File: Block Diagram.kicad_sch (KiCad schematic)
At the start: 0 parts

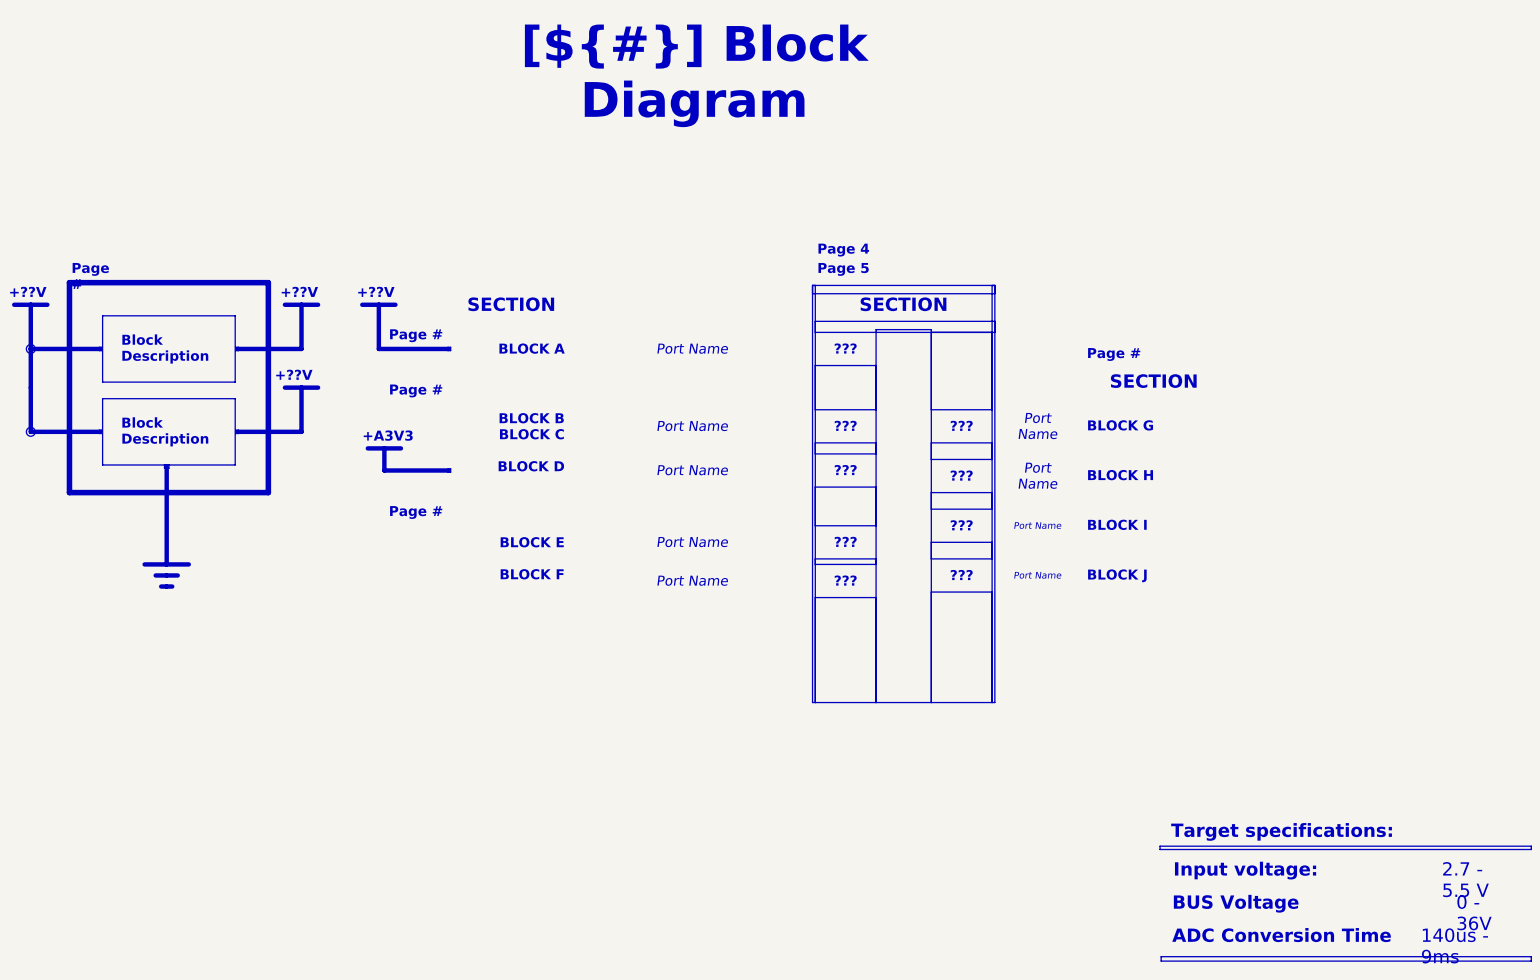
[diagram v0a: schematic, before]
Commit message: Outputs generated, ready for prototyping
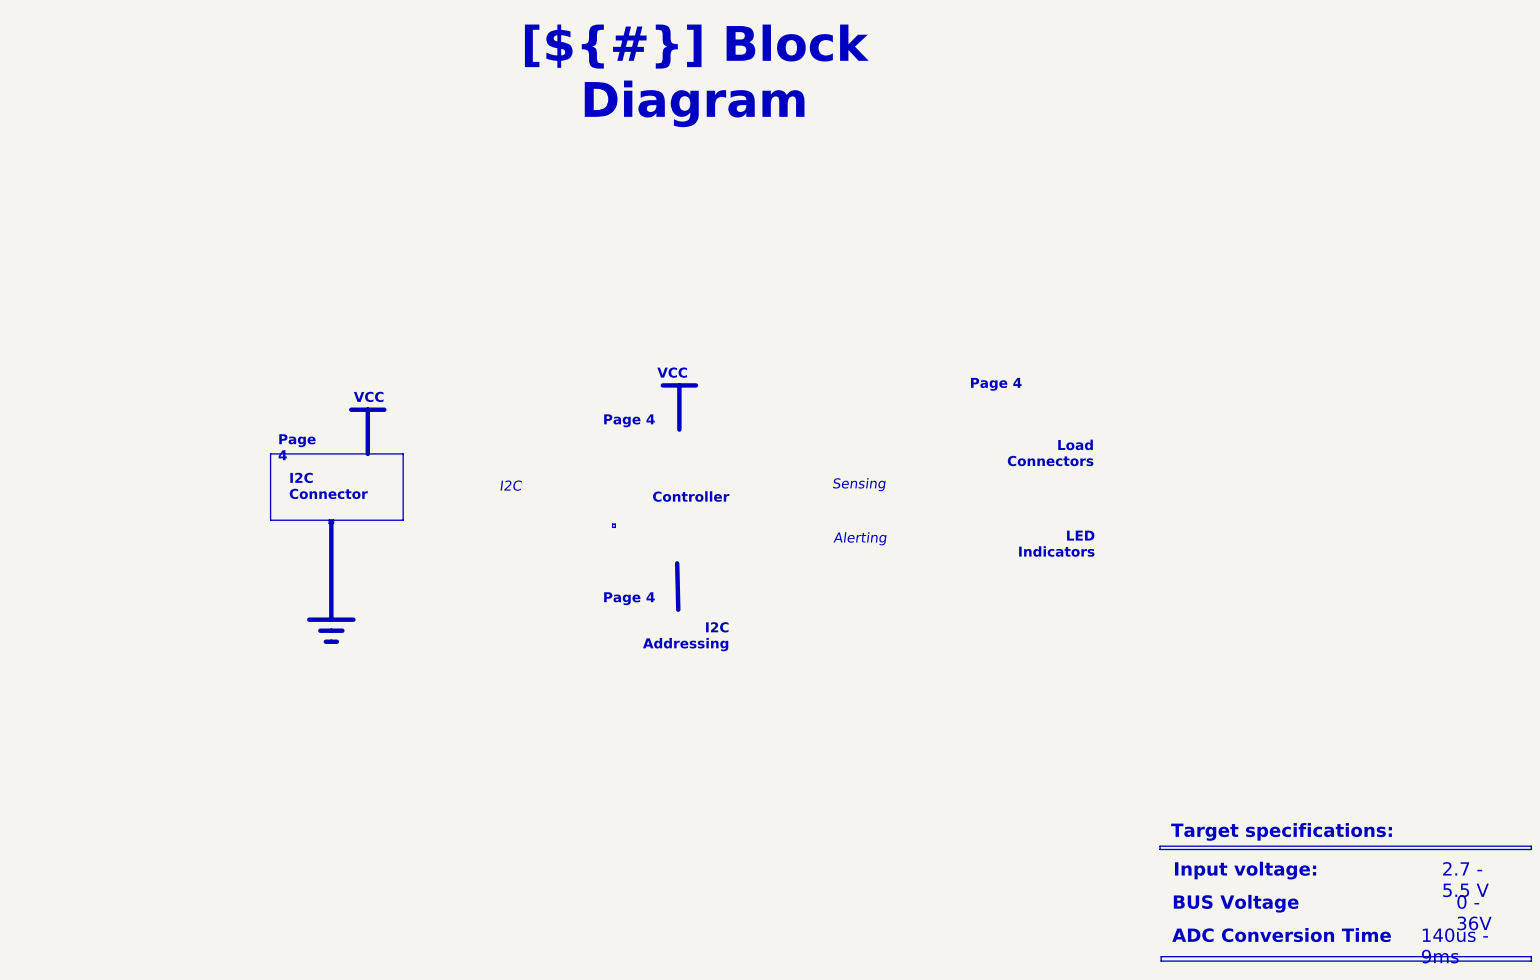
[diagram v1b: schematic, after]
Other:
- note added: "VCC"
- note removed: "+??V"
- note removed: "+A3V3"
